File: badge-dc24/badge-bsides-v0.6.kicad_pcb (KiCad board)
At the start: 2 copper layers, 50 parts, among them P1 USB_OTG, P2 CONN_01X04, U1 ESP-12E, U2 TSOP38238, U3 74HC595, U4 MC78L05ACH, U5 74LS165

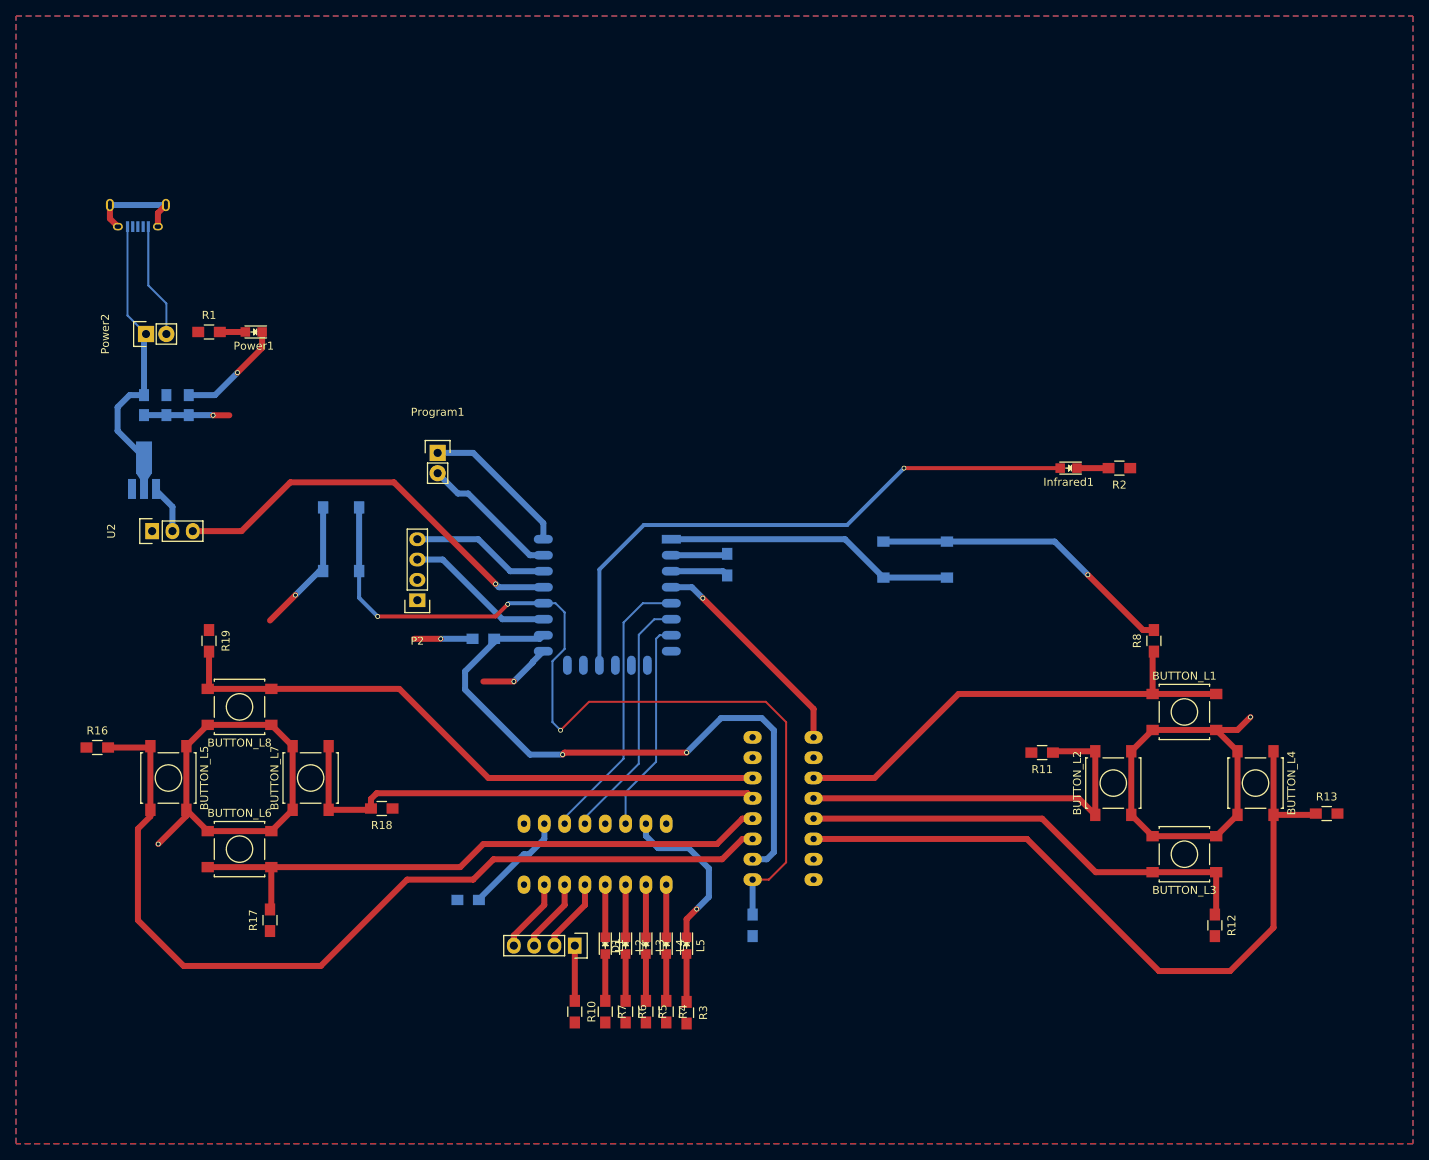
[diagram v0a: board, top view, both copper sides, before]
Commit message: last v0.6
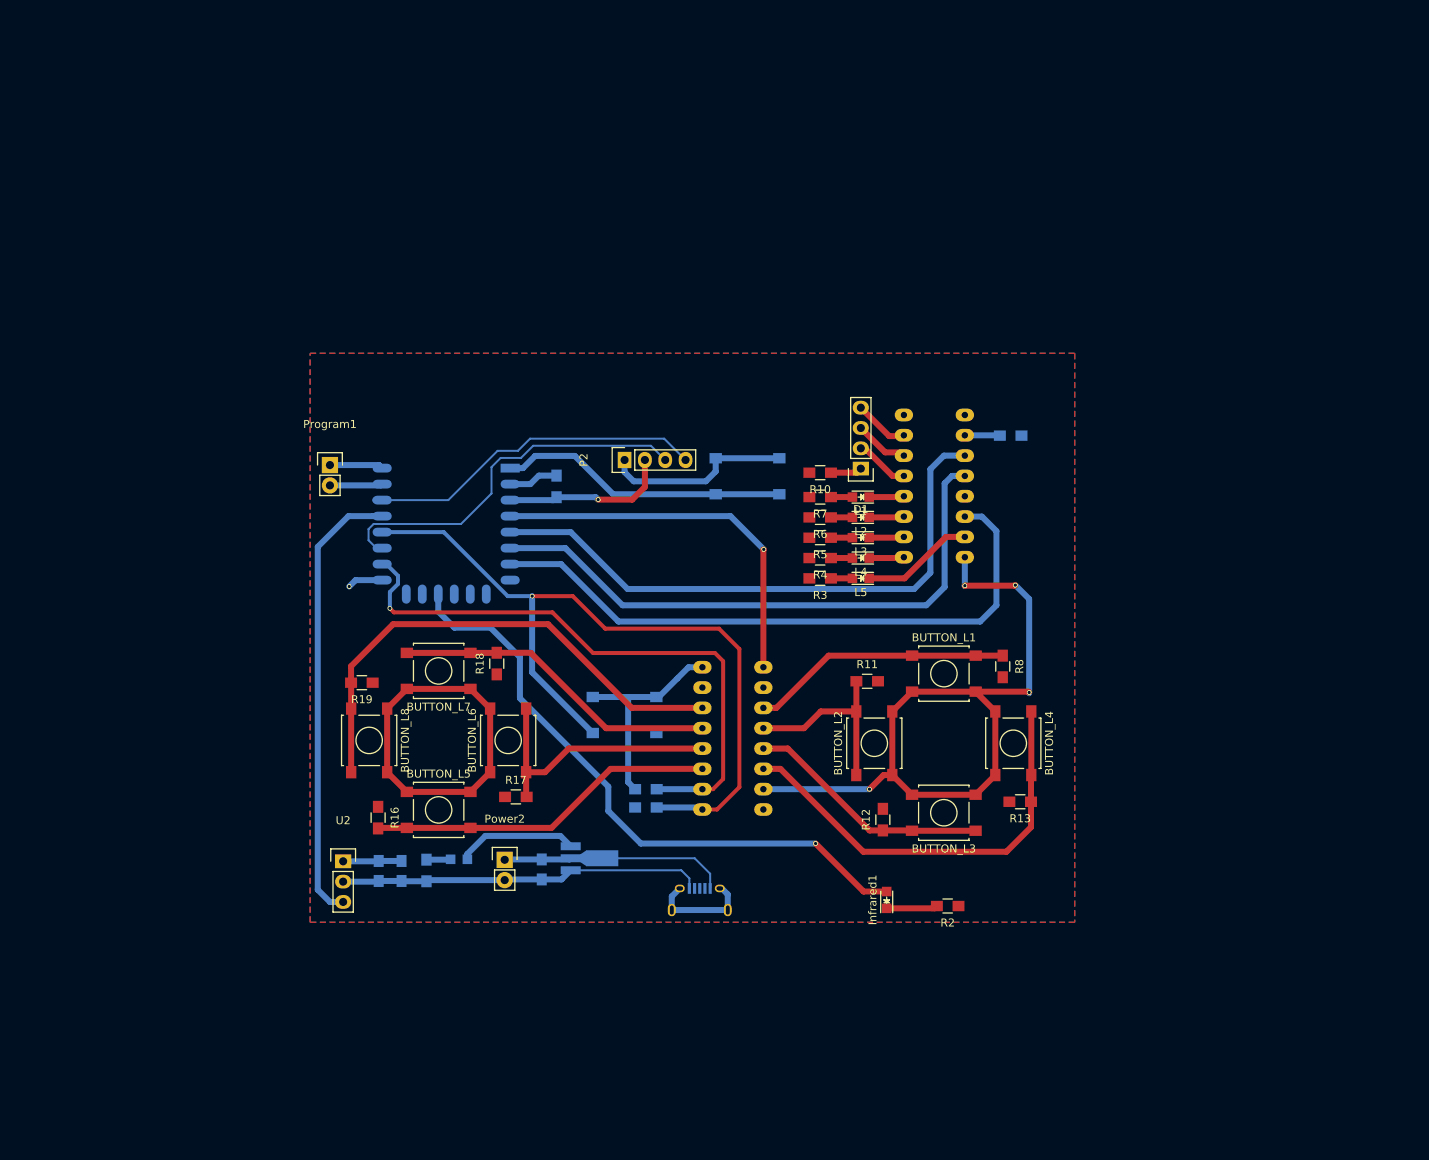
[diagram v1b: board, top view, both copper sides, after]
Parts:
- Power1, R1: moved to B.Cu
- moved P1 110.9 mm to (100.7, 126.5), turned to 180 degrees
- moved R9 89.3 mm to (139.6, 68.3), turned to 0 degrees
- moved Power2 79.6 mm to (76.3, 121.3), turned to 0 degrees
- moved C2 76.4 mm to (81.0, 122.6)
- moved R10 74.0 mm to (115.8, 73.0), turned to 180 degrees
- moved U4 73.9 mm to (86.9, 121.2), turned to 90 degrees
- moved R1 72.6 mm to (66.5, 122.7), turned to 90 degrees
- moved Power1 70.7 mm to (70.6, 121.3)
- moved R7 69.7 mm to (115.8, 76.0), turned to 180 degrees
- moved D1 69.5 mm to (120.8, 72.5), turned to 180 degrees
- moved R6 66.4 mm to (115.8, 78.5), turned to 180 degrees
- moved C3 65.2 mm to (63.4, 122.7)
- moved L1 64.5 mm to (120.8, 76.0), turned to 180 degrees
- moved R5 63.1 mm to (115.8, 81.1), turned to 180 degrees
- moved C1 62.9 mm to (60.6, 122.7)
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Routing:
- net Net-(BUTTON_L5-Pad2): track 113.8 -> 43.6 mm
- net +3V3: track 125.3 -> 182.8 mm, vias 3 -> 5
- net Net-(U1-Pad7): track 26.8 -> 78.6 mm
- net Net-(U1-Pad6): track 31.3 -> 74.1 mm
- net Net-(BUTTON_L6-Pad2): track 76.0 -> 34.3 mm
- net Net-(BUTTON_L4-Pad1): track 94.0 -> 53.5 mm
- net Net-(U1-Pad5): track 35.2 -> 74.3 mm
- net Net-(P2-Pad3): track 18.8 -> 48.6 mm
- net Net-(BUTTON_L3-Pad1): track 58.5 -> 30.8 mm
- net Net-(BUTTON_L1-Pad1): track 60.0 -> 32.8 mm
- net Net-(P2-Pad4): track 17.4 -> 43.1 mm
- net Net-(BUTTON_L2-Pad1): track 49.4 -> 24.2 mm
- net Net-(BUTTON_L7-Pad2): track 62.8 -> 40.9 mm
- net Net-(U1-Pad4): track 27.6 -> 48.2 mm
- net Net-(BUTTON_L8-Pad2): track 77.7 -> 63.7 mm
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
